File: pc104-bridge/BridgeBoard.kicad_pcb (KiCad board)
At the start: 2 copper layers, 73.7 x 34.3 mm, 2 parts

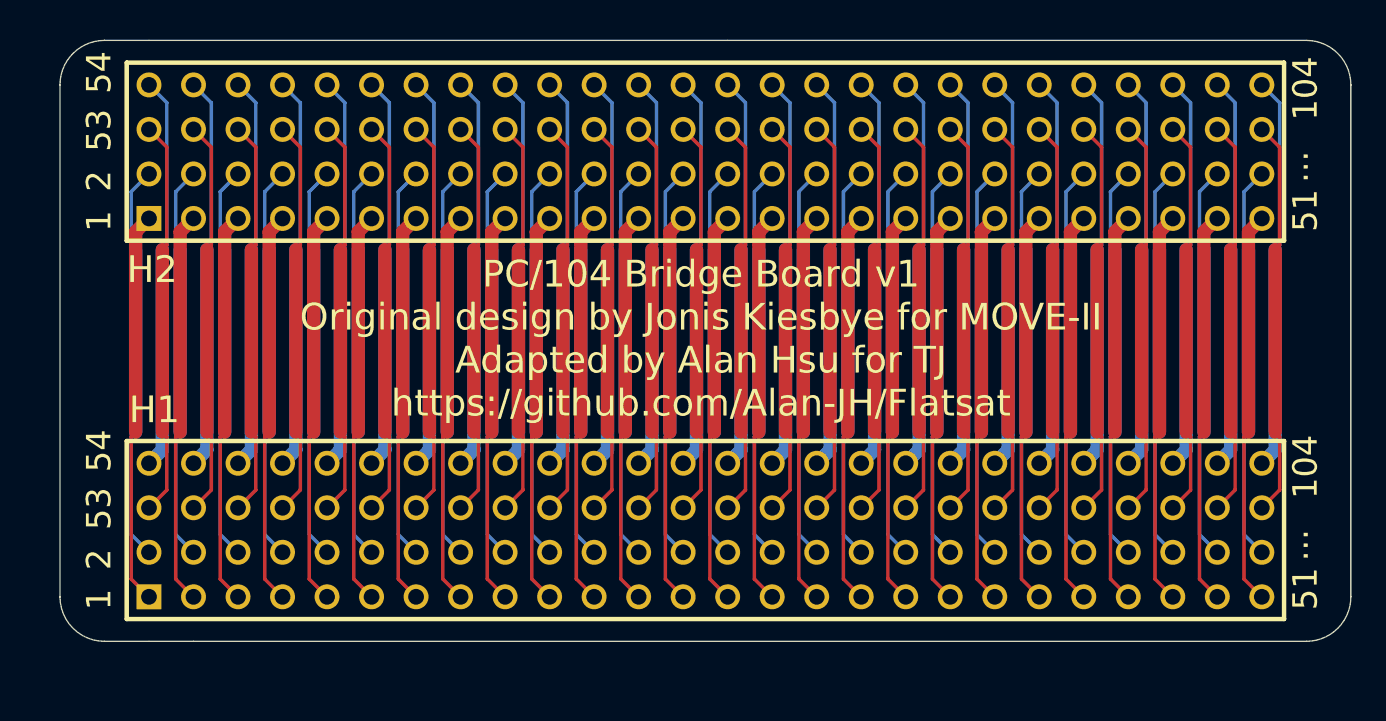
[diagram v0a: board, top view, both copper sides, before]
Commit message: fix board edge
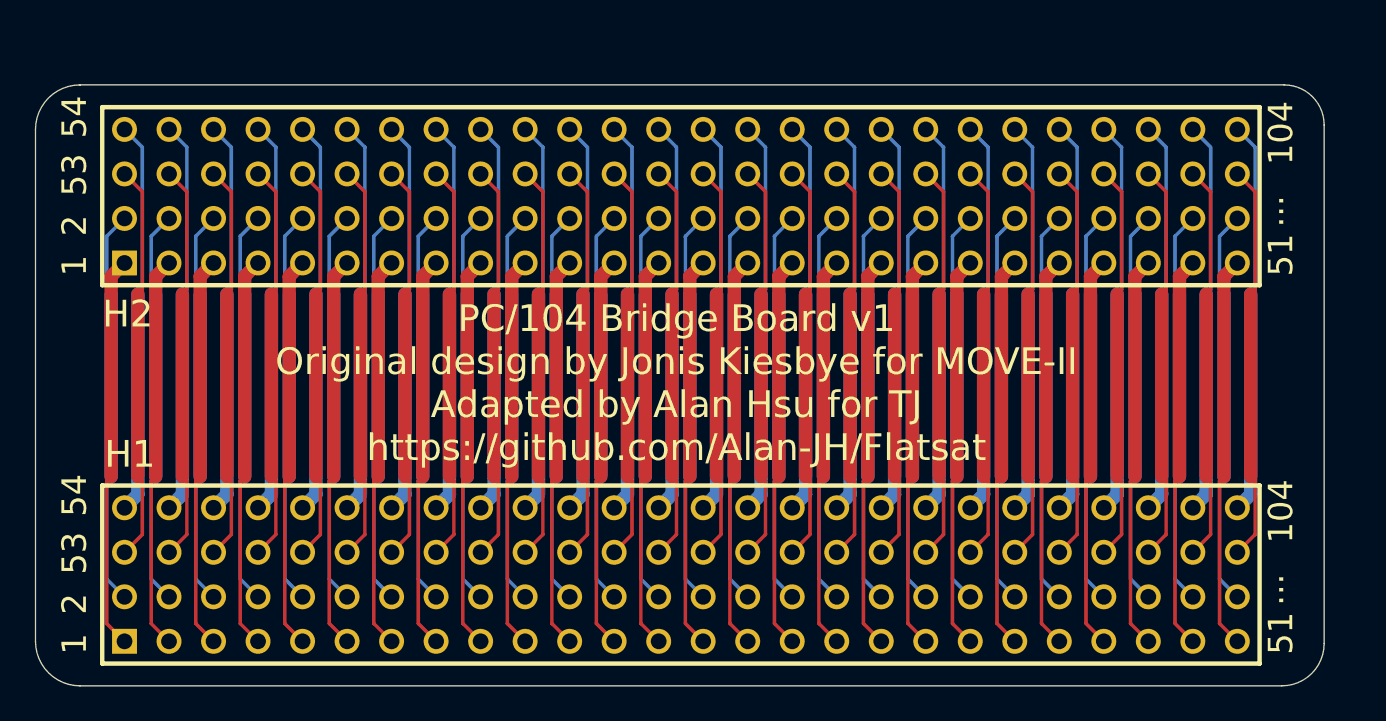
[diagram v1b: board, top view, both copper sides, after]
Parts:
- moved H1 2.90 mm to (115.4, 122.1)
- moved H2 2.90 mm to (115.4, 100.6)
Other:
- board size 73.7 x 34.3 mm -> 73.5 x 34.3 mm
